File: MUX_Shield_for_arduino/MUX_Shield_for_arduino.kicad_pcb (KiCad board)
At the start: 2 copper layers, 58.4 x 93.3 mm, 32 parts, among them J1 CONN_05X20.05_IN_PTH_SILK, J2 CONN_05X20.05_IN_PTH_SILK, J3 CONN_05X20.05_IN_PTH_SILK, J4 CONN_05X20.05_IN_PTH_SILK, J5 CONN_05X20.05_IN_PTH_SILK, J6 CONN_05X20.05_IN_PTH_SILK, J7 CONN_05X20.05_IN_PTH_SILK, J8 CONN_05X20.05_IN_PTH_SILK, J9 CONN_06X2PTH_FEMALE, U1 74HC4067SM96, U2 74HC4067SM96, U3 74HC4067SM96, U4 74HC4067SM96, U5 MCP23S08

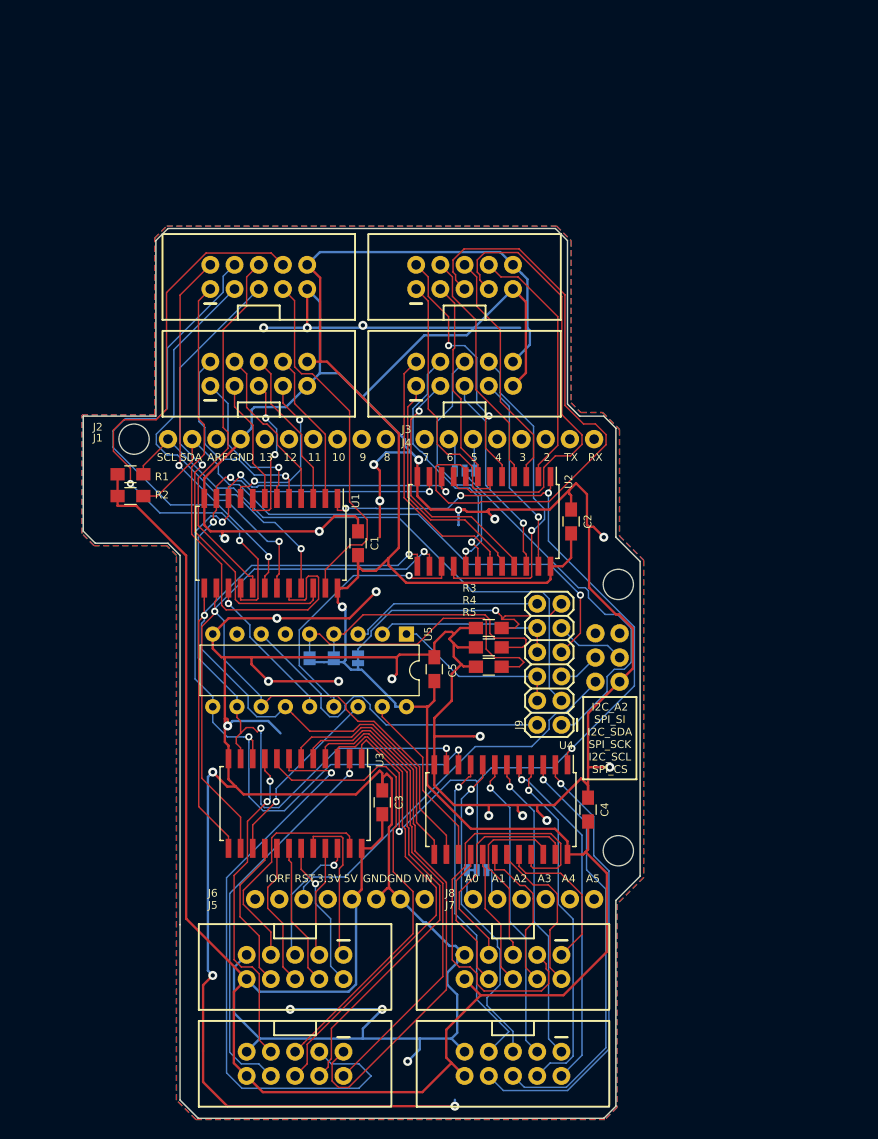
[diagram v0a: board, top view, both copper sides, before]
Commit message: add buttons and pots sub-boards, push changes
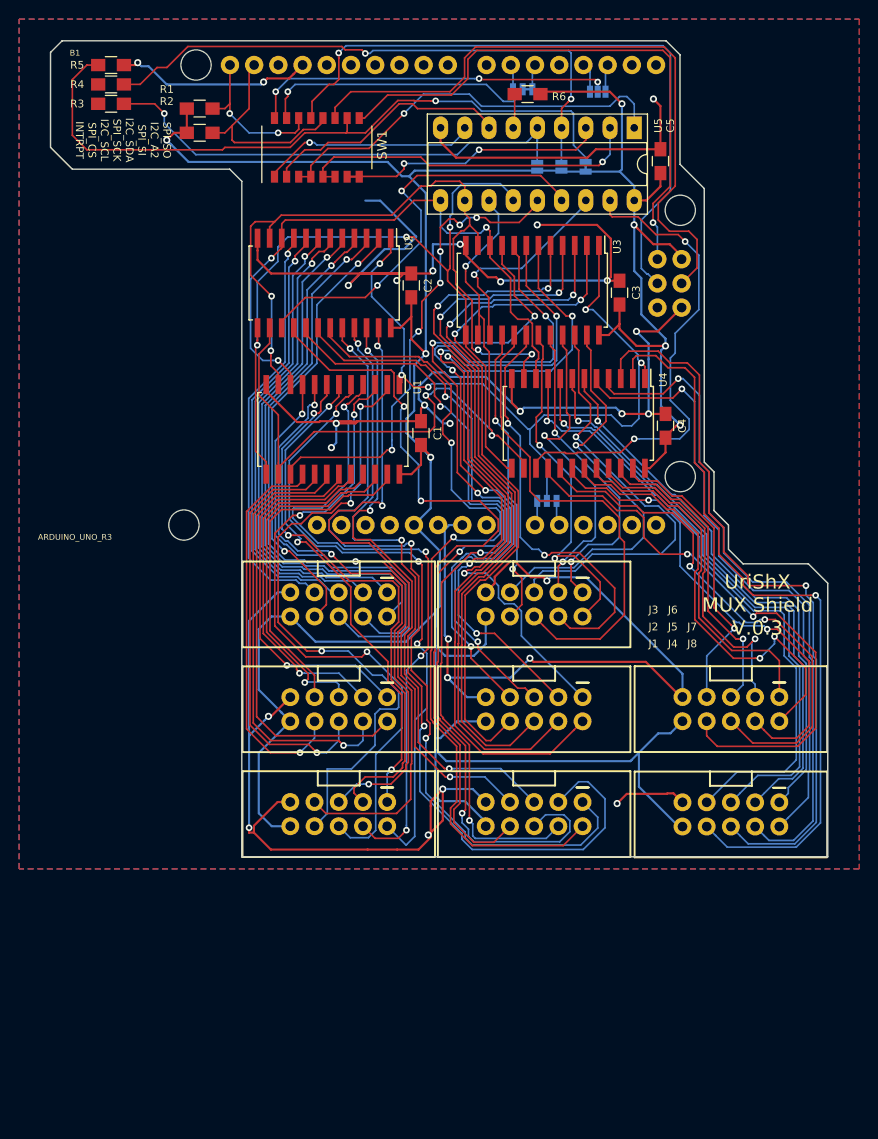
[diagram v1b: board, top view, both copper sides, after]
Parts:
- removed J9: CONN_06X2PTH_FEMALE, SparkFun Connectors:2X6
- removed SYMBOL1: KiCad-Logo2_6mm_SilkScreen, Symbols:KiCad-Logo2_6mm_SilkScreen
- removed SYMBOL2: OSHW-Symbol_6.7x6mm_SilkScreen, Symbols:OSHW-Symbol_6.7x6mm_SilkScreen
- added JP6: INT, SparkFun Jumpers:SMT-JUMPER_3_NO_SILK, B.Cu at (153.7, 61.2)
- added R6: 10K, Resistors_SMD:R_0805_HandSoldering, F.Cu at (146.3, 61.5)
- added SW1: SW_DIP_x08, Buttons_Switches_SMD:SW_DIP_x8_W6.15mm_Slide_Omron_A6H, F.Cu at (124.2, 67.1)
- J1, J2, J3, J4, J5, J6, J7, J8: footprint SparkFun Connectors:2X5-SHROUDED -> MyFootprintLib:2X5-SHROUDED
- U5: footprint Housings_DIP:DIP-18_W7.62mm -> Housings_DIP:DIP-18_W7.62mm_Socket_LongPads
- moved R4 71.1 mm to (102.6, 60.5)
- moved R5 71.1 mm to (102.6, 62.5)
- moved R3 71.1 mm to (102.6, 58.4), turned to 0 degrees
- moved U3 59.3 mm to (146.8, 82.0)
- moved C3 59.0 mm to (156.0, 82.3)
- moved C5 58.3 mm to (160.2, 68.5)
- moved U5 58.2 mm to (157.5, 65.0)
- moved JP1 56.8 mm to (152.4, 69.1)
- moved JP2 56.8 mm to (149.9, 69.1)
- moved JP3 56.8 mm to (147.3, 69.1)
- moved J1 47.0 mm to (126.5, 137.0), turned to 270 degrees
- moved J4 46.8 mm to (147.0, 137.0), turned to 270 degrees
- moved J2 46.1 mm to (126.5, 126.0), turned to 270 degrees
- moved J6 45.6 mm to (147.0, 115.0)
- moved J5 44.9 mm to (147.0, 126.0)
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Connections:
- net Net-(B1-PadSCL) renamed /SCL
- net Net-(B1-PadSDA) renamed /SDA
- net Net-(J9-Pad11) renamed /I2C_A2
- B1 pad 3.3V: (no net) -> Net-(B1-Pad3.3V)
- B1 pad A2: (no net) -> Net-(B1-PadA2)
- B1 pad A3: (no net) -> Net-(B1-PadA3)
- B1 pad A4: (no net) -> Net-(B1-PadA4)
- B1 pad A5: (no net) -> Net-(B1-PadA5)
- B1 pad AREF: (no net) -> Net-(B1-PadAREF)
- B1 pad D0: (no net) -> Net-(B1-PadD0)
- B1 pad D1: (no net) -> Net-(B1-PadD1)
- B1 pad D10: (no net) -> Net-(B1-PadD10)
- B1 pad D11: (no net) -> Net-(B1-PadD11)
- B1 pad D12: (no net) -> Net-(B1-PadD12)
- B1 pad D13: (no net) -> Net-(B1-PadD13)
- B1 pad D2: (no net) -> Net-(B1-PadD2)
- B1 pad D3: (no net) -> Net-(B1-PadD3)
- B1 pad D4: (no net) -> Net-(B1-PadD4)
- B1 pad D7: (no net) -> Net-(B1-PadD7)
- B1 pad D8: (no net) -> Net-(B1-PadD8)
- B1 pad D9: (no net) -> Net-(B1-PadD9)
- B1 pad IORE: (no net) -> Net-(B1-PadIORE)
- B1 pad MISO: (no net) -> /MISO
- B1 pad MOSI: Net-(B1-PadMOSI) -> /MOSI
- B1 pad SCK: Net-(B1-PadSCK) -> /SCK
- B1 pad VCC: (no net) -> VCC
- B1 pad VIN: (no net) -> Net-(B1-PadVIN)
- JP4 pad 2: Net-(J9-Pad1) -> /~CS
- U5 pad 6: (no net) -> Net-(R6-Pad2)
- U5 pad 8: (no net) -> Net-(SW1-Pad1)
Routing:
- net GND: track 521.6 -> 377.4 mm, vias 29 -> 27
- net /SCK: track 0.00 -> 70.6 mm, vias 0 -> 1
- net /MOSI: track 0.00 -> 69.0 mm
- net Net-(J4-Pad6): track 26.4 -> 92.2 mm, vias 1 -> 3
- net Net-(J4-Pad3): track 27.1 -> 89.8 mm, vias 1 -> 3
- net Net-(J4-Pad2): track 27.7 -> 90.0 mm, vias 0 -> 2
- net Net-(J4-Pad1): track 25.5 -> 87.0 mm, vias 0 -> 3
- net /MISO: track 0.00 -> 59.2 mm, vias 0 -> 1
- net Net-(J4-Pad4): track 27.0 -> 84.0 mm, vias 1 -> 3
- net Net-(J1-Pad4): track 17.5 -> 70.5 mm, vias 0 -> 4
- net Net-(J1-Pad6): track 16.7 -> 69.3 mm, vias 0 -> 3
- net Net-(J1-Pad8): track 16.2 -> 68.7 mm, vias 0 -> 3
- net Net-(J1-Pad7): track 18.0 -> 67.5 mm
- net Net-(J4-Pad7): track 21.1 -> 68.3 mm, vias 1 -> 3
- net Net-(J1-Pad3): track 13.1 -> 59.9 mm, vias 0 -> 2
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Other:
- board size 58.4 x 93.3 mm -> 81.5 x 85.6 mm
- net class Default: trace_width 0.1524 -> 0.175; via_dia 0.762 -> 0.7; via_drill 0.4064 -> 0.35
- net class PWR: trace_width 0.25 -> 0.225; via_dia 0.95 -> 0.75; via_drill 0.45 -> 0.4
- rule via_min_drill: 0.35 -> 0.3
- rule via_min_size: 0.6858 -> 0.65
- board text added: "SPI_SO I2C_A2 SPI_SI I2C_SDA SPI_SCK I2C_SCL SPI_CS INTRPT"
- board text added: "UriShX MUX Shield V.0.3"
- board text removed: "I2C_A2 SPI_SI I2C_SDA SPI_SCK I2C_SCL SPI_CS"
